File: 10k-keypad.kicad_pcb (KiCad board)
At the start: 2 copper layers, 107.2 x 55.2 mm, 39 parts, among them J1 AVR-ISP-6, K1 SW_Push, K10 SW_Push, K2 SW_Push, K3 SW_Push, K4 SW_Push, K5 SW_Push, K6 SW_Push, K7 SW_Push, K8 SW_Push, K9 SW_Push, SW1 SW_Push, U1 ATmega16U2-A, Y1 Crystal_GND24_Small

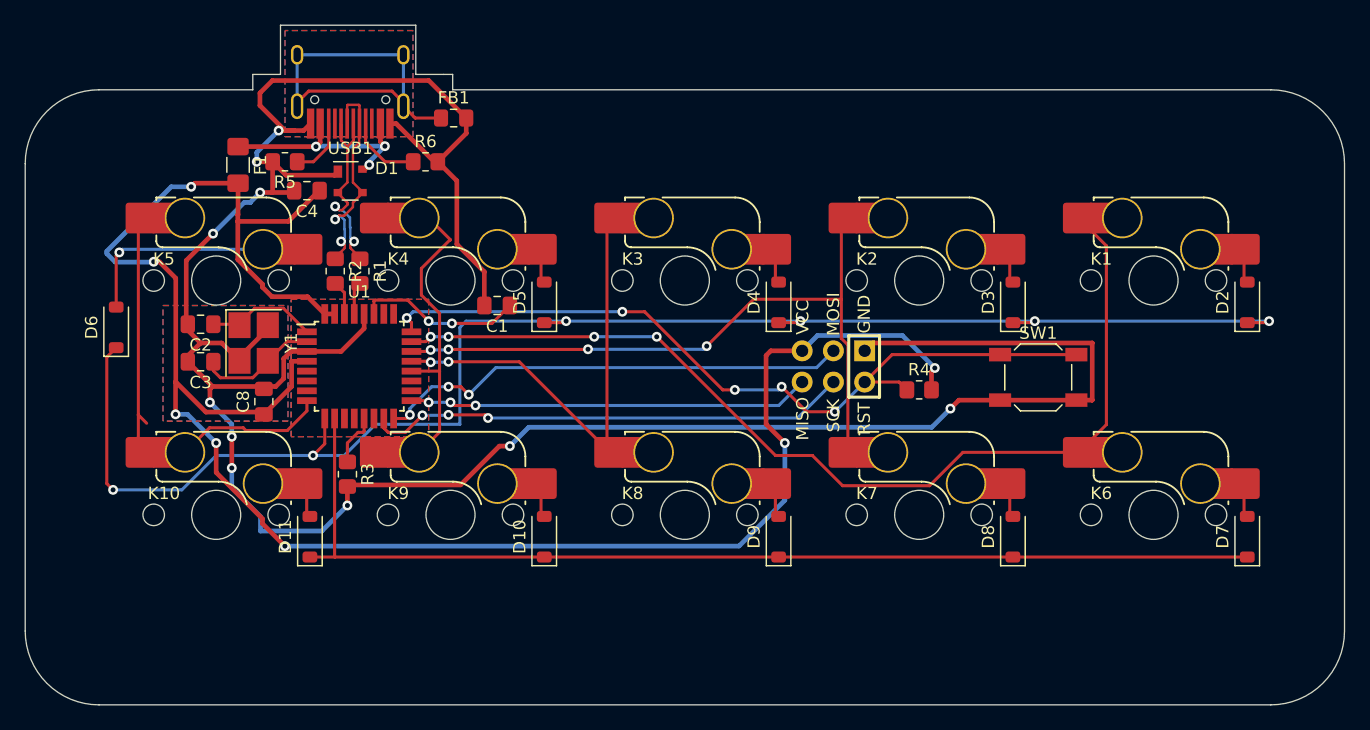
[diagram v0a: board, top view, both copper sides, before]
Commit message: hall sensor circuitry
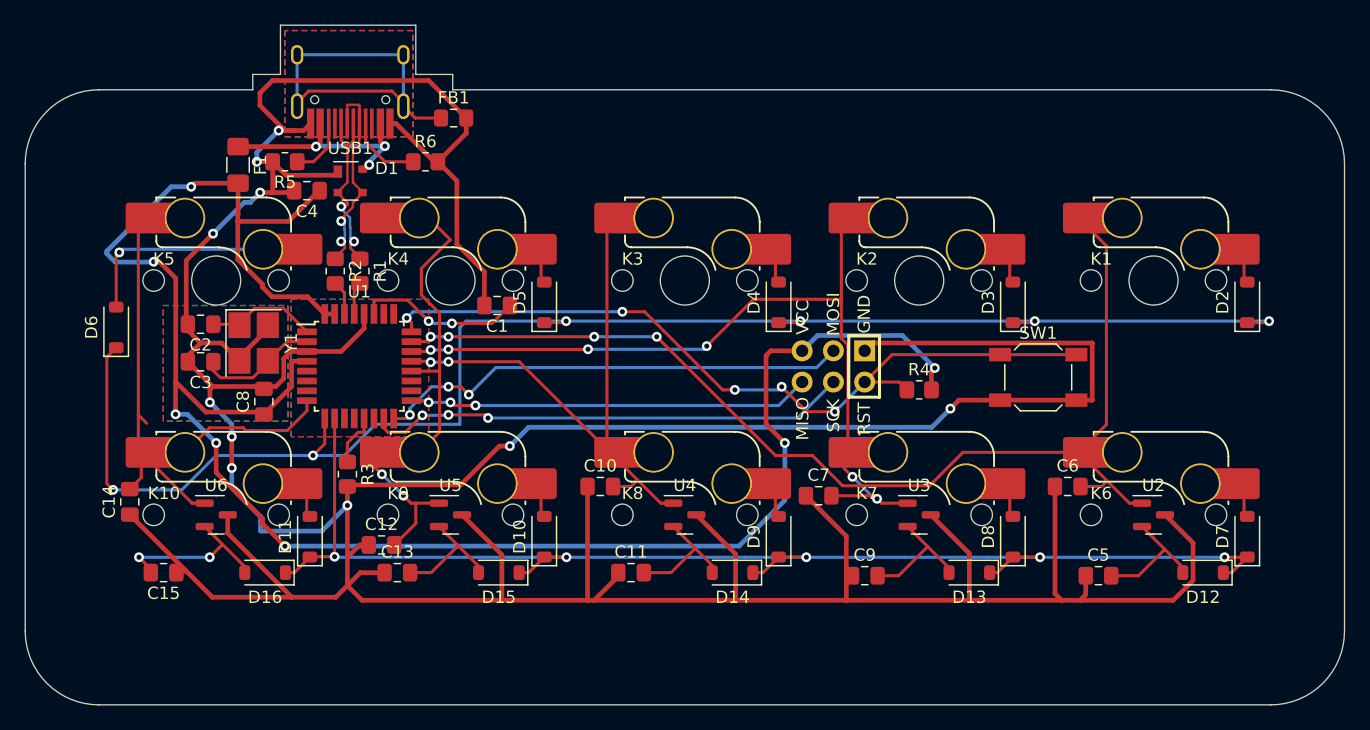
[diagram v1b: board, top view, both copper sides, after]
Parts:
- added C10: 100n, Capacitor_SMD:C_0805_2012Metric_Pad1.18x1.45mm_HandSolder, F.Cu at (150.8, 78.5)
- added C11: 4.7n, Capacitor_SMD:C_0805_2012Metric_Pad1.18x1.45mm_HandSolder, F.Cu at (153.2, 85.5)
- added C12: 100n, Capacitor_SMD:C_0805_2012Metric_Pad1.18x1.45mm_HandSolder, F.Cu at (133.0, 83.2)
- added C13: 4.7n, Capacitor_SMD:C_0805_2012Metric_Pad1.18x1.45mm_HandSolder, F.Cu at (134.2, 85.5)
- added C14: 100n, Capacitor_SMD:C_0805_2012Metric_Pad1.18x1.45mm_HandSolder, F.Cu at (112.5, 79.8)
- added C15: 4.7n, Capacitor_SMD:C_0805_2012Metric_Pad1.18x1.45mm_HandSolder, F.Cu at (115.2, 85.5)
- added C5: 4.7n, Capacitor_SMD:C_0805_2012Metric_Pad1.18x1.45mm_HandSolder, F.Cu at (191.2, 85.8)
- added C6: 100n, Capacitor_SMD:C_0805_2012Metric_Pad1.18x1.45mm_HandSolder, F.Cu at (188.8, 78.5)
- added C7: 100n, Capacitor_SMD:C_0805_2012Metric_Pad1.18x1.45mm_HandSolder, F.Cu at (168.5, 79.2)
- added C9: 4.7n, Capacitor_SMD:C_0805_2012Metric_Pad1.18x1.45mm_HandSolder, F.Cu at (172.2, 85.8)
- added D12: D, Diode_SMD:D_SOD-123, F.Cu at (199.8, 85.5)
- added D13: D, Diode_SMD:D_SOD-123, F.Cu at (180.8, 85.5)
- added D14: D, Diode_SMD:D_SOD-123, F.Cu at (161.5, 85.5)
- added D15: D, Diode_SMD:D_SOD-123, F.Cu at (142.5, 85.5)
- added D16: D, Diode_SMD:D_SOD-123, F.Cu at (123.5, 85.5)
- added U2: DRV5055A2xDBZxQ1, Package_TO_SOT_SMD:SOT-23, F.Cu at (195.7, 80.8)
- added U3: DRV5055A2xDBZxQ1, Package_TO_SOT_SMD:SOT-23, F.Cu at (176.7, 80.8)
- added U4: DRV5055A2xDBZxQ1, Package_TO_SOT_SMD:SOT-23, F.Cu at (157.6, 80.8)
- added U5: DRV5055A2xDBZxQ1, Package_TO_SOT_SMD:SOT-23, F.Cu at (138.6, 80.8)
- added U6: DRV5055A2xDBZxQ1, Package_TO_SOT_SMD:SOT-23, F.Cu at (119.5, 80.8)
- K10, K6, K7, K8, K9: footprint marbastlib-mx:SW_MX_HS_CPG151101S11_1u -> Hall:SW_MX_HS_CPG151101S11_1u_no_center_piece
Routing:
- net GND: track 218.7 -> 396.7 mm
- net ROW2: track 87.5 -> 106.4 mm, vias 0 -> 5
- net Net-(D16-A): track 0.00 -> 14.0 mm, vias 0 -> 2
- net COL4: track 28.7 -> 40.4 mm, vias 0 -> 2
- net COL2: track 56.2 -> 67.6 mm, vias 4 -> 6
- net Net-(D13-A): track 0.00 -> 10.6 mm
- net Net-(D12-A): track 0.00 -> 10.4 mm
- net COL5: track 32.5 -> 42.8 mm
- net Net-(D14-A): track 0.00 -> 10.0 mm
- net Net-(D15-A): track 0.00 -> 9.89 mm
- net COL1: track 81.5 -> 90.7 mm
- net COL3: track 38.5 -> 47.6 mm
- net D-: track 18.8 -> 17.5 mm
- net D+: track 16.9 -> 15.8 mm
